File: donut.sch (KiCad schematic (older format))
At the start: 39 parts, among them J1 AVRISP6, J2 Jack, P1 PAD1, P2 PAD2, P3 PAD2, P4 PAD1, P5 PAD2, P6 PAD2, SW1 S0, SW10 TACTILE, SW11 TACTILE, SW12 TACTILE, SW13 MODE, SW14 TACTILE, SW2 TACTILE, SW3 TACTILE, SW4 TACTILE, SW5 TACTILE, SW6 TACTILE, SW7 TACTILE, SW8 TACTILE, SW9 TACTILE, U1 ATMEGA48PA-MU, X1 XTAL4P

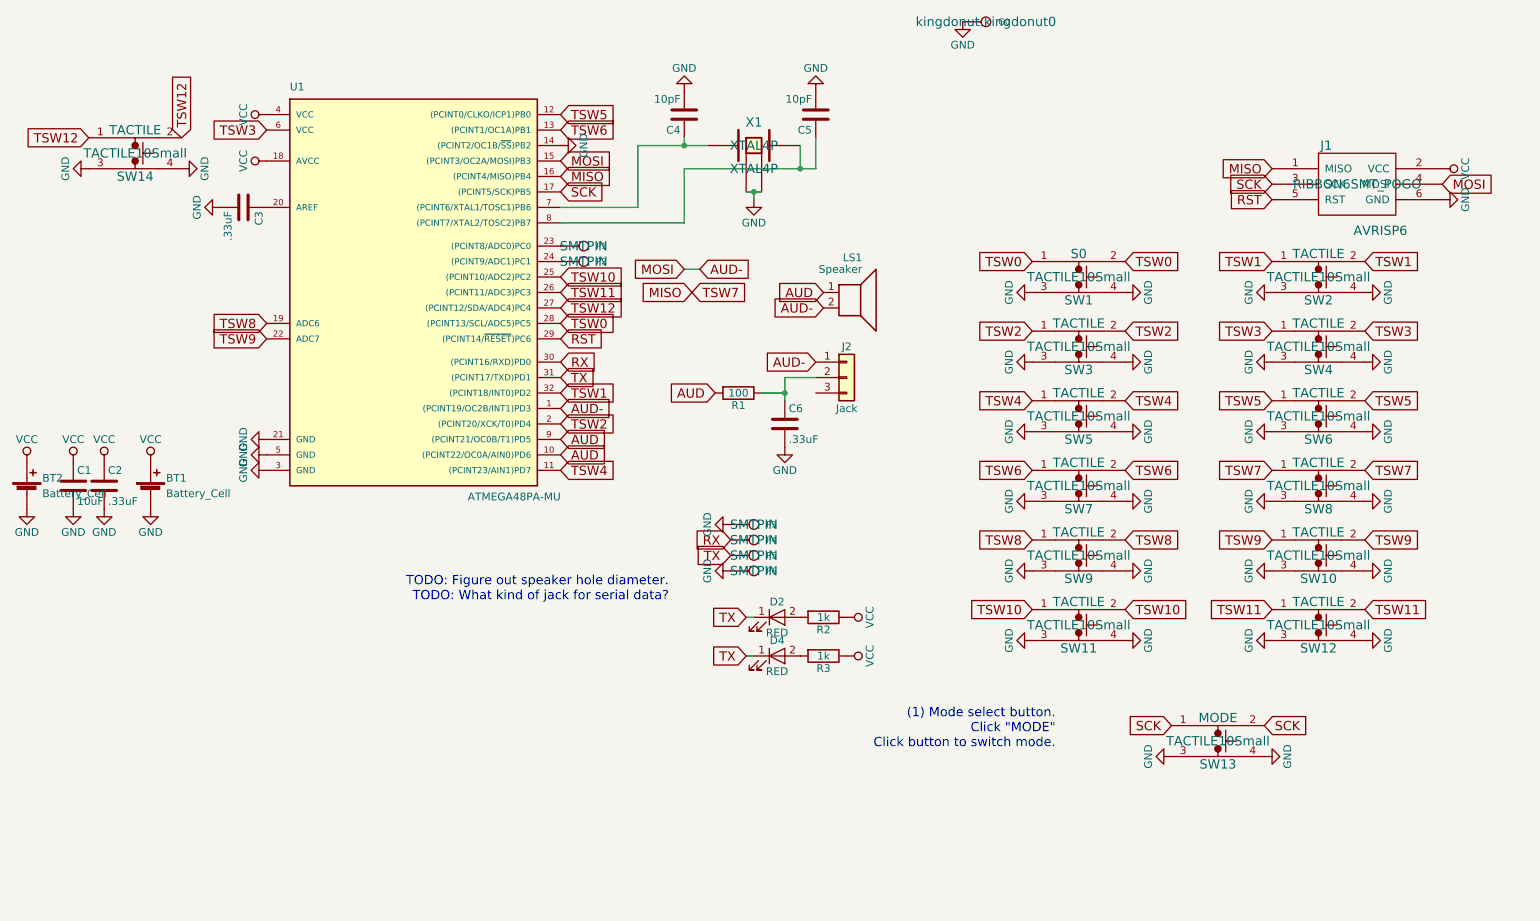
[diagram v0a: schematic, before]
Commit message: Update
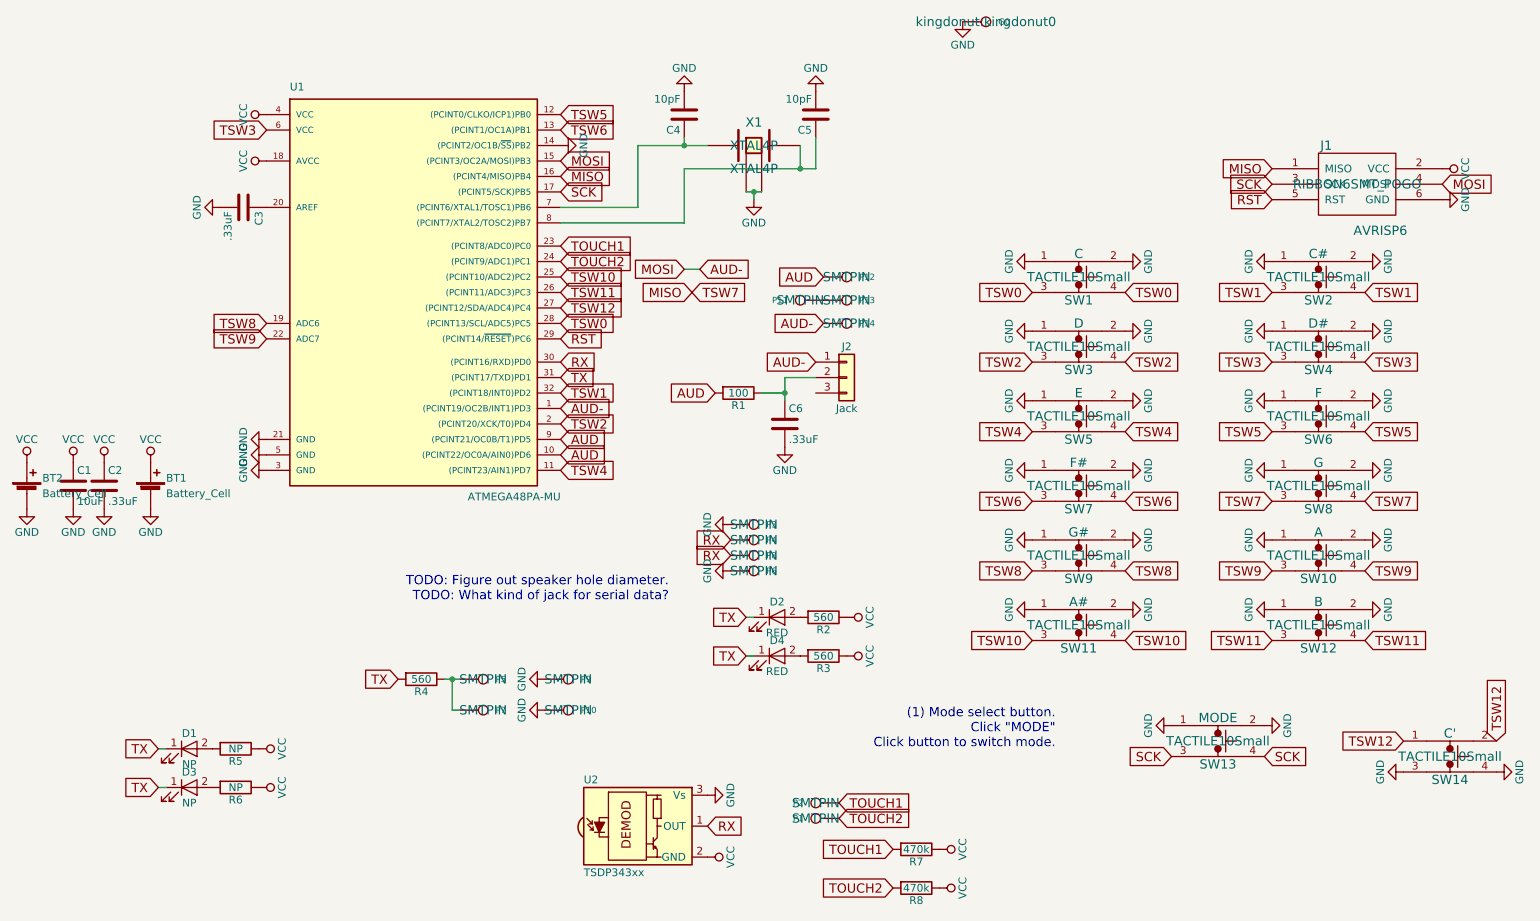
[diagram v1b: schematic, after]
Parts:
- removed LS1: Speaker, S8211-45R, symbol Speaker
- added D1, D3: NP, LED_0603, symbol LED
- added P10, P11, P12, P13, P14, P7, P9: PAD2, SMTPIN, symbol CONN_1
- added P8: PAD1, SMTPIN, symbol CONN_1
- added R4: 560, R_0805, symbol R
- added R5, R6: NP, R_0805, symbol R
- added R7, R8: 470k, R_0805, symbol R
- added U2: TSDP343xx, TO-92_Inline_Narrow_Oval, symbol TSDP343xx
- R2, R3: value 1k -> 560
- SW1: value S0 -> C
- SW10: value TACTILE -> A
- SW11: value TACTILE -> A#
- SW12: value TACTILE -> B
- SW14: value TACTILE -> C'
- SW2: value TACTILE -> C#
- SW3: value TACTILE -> D
- SW4: value TACTILE -> D#
- SW5: value TACTILE -> E
- SW6: value TACTILE -> F
- SW7: value TACTILE -> F#
- SW8: value TACTILE -> G
- SW9: value TACTILE -> G#
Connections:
- net AUD: now also P12.1
- net AUD-: now also P14.1
- net GND: now also SW1.1, SW1.2, SW10.1, SW10.2, SW11.1, SW11.2, SW12.1, SW12.2, SW13.1, SW13.2, SW2.1, SW2.2, SW3.1, SW3.2, SW4.1, SW4.2, SW5.1, SW5.2, SW6.1, SW6.2, SW7.1, SW7.2, SW8.1, SW8.2, SW9.1, SW9.2, P10.1, P9.1, U2.3 (Vs); no longer SW1.3, SW1.4, SW10.3, SW10.4, SW11.3, SW11.4, SW12.3, SW12.4, SW13.3, SW13.4, SW2.3, SW2.4, SW3.3, SW3.4, SW4.3, SW4.4, SW5.3, SW5.4, SW6.3, SW6.4, SW7.3, SW7.4, SW8.3, SW8.4, SW9.3, SW9.4
- net MISO: now also SW8.3, SW8.4; no longer SW8.1, SW8.2
- net RX: now also P8.1, U2.1 (OUT)
- net SCK: now also SW13.3, SW13.4; no longer SW13.1, SW13.2
- net TSW0: now also SW1.3, SW1.4; no longer SW1.1, SW1.2
- net TSW1: now also SW2.3, SW2.4; no longer SW2.1, SW2.2
- net TSW10: now also SW11.3, SW11.4; no longer SW11.1, SW11.2
- net TSW11: now also SW12.3, SW12.4; no longer SW12.1, SW12.2
- net TSW2: now also SW3.3, SW3.4; no longer SW3.1, SW3.2
- net TSW3: now also SW4.3, SW4.4; no longer SW4.1, SW4.2
- net TSW4: now also SW5.3, SW5.4; no longer SW5.1, SW5.2
- net TSW5: now also SW6.3, SW6.4; no longer SW6.1, SW6.2
- net TSW6: now also SW7.3, SW7.4; no longer SW7.1, SW7.2
- net TSW8: now also SW9.3, SW9.4; no longer SW9.1, SW9.2
- net TSW9: now also SW10.3, SW10.4; no longer SW10.1, SW10.2
- net TX: now also D1.1 (K), D3.1 (K), R4.2; no longer P5.1
- net VCC: now also R5.1, R6.1, R7.1, R8.1, U2.2 (GND)
- net TOUCH1: now reaches U1.23 ((PCINT8/ADC0)PC0)
- net TOUCH1: now also P2.1, R7.2; no longer P1.1
- net TOUCH2: now reaches U1.24 ((PCINT9/ADC1)PC1)
- net TOUCH2: now also P1.1, R8.2; no longer P2.1
- new net: P5.1, P7.1, R4.1
- new net: P11.1, P13.1
- new net: D1.2 (A), R5.2
- new net: D3.2 (A), R6.2
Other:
- moved on the sheet: P1, P2, P5, SW14
